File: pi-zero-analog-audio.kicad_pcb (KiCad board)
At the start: 2 copper layers, 65 x 30 mm, 40 parts, among them J1 GPIO, J2 Screw_Terminal_01x04, J3 Audio Jack, U1 MIC5365-3.3YD5, U2 MC74VHC1GT50, U3 MC74VHC1GT50, U4 PAM8403D

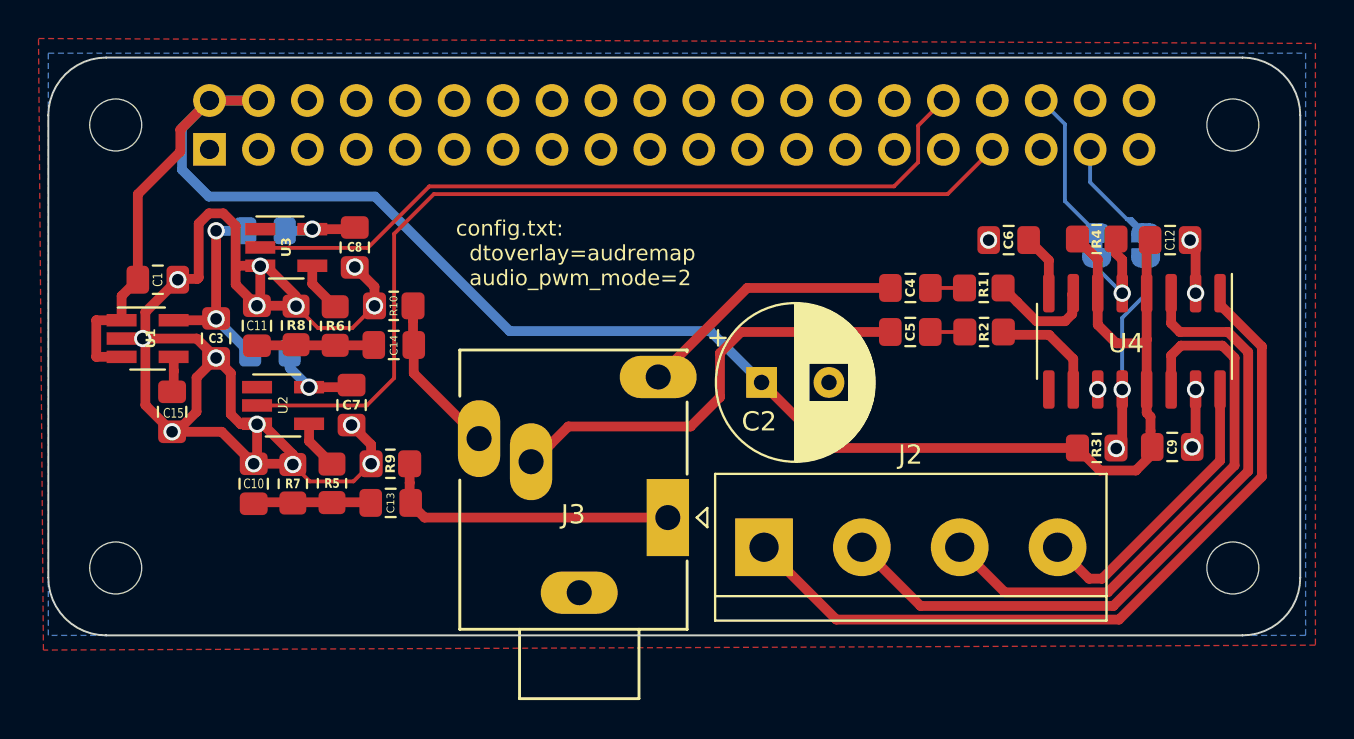
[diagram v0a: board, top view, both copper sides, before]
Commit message: Revert "Two GND zones"
This reverts commit edaad1ef0305b16592a24cacb57811a0cb0df8b8.
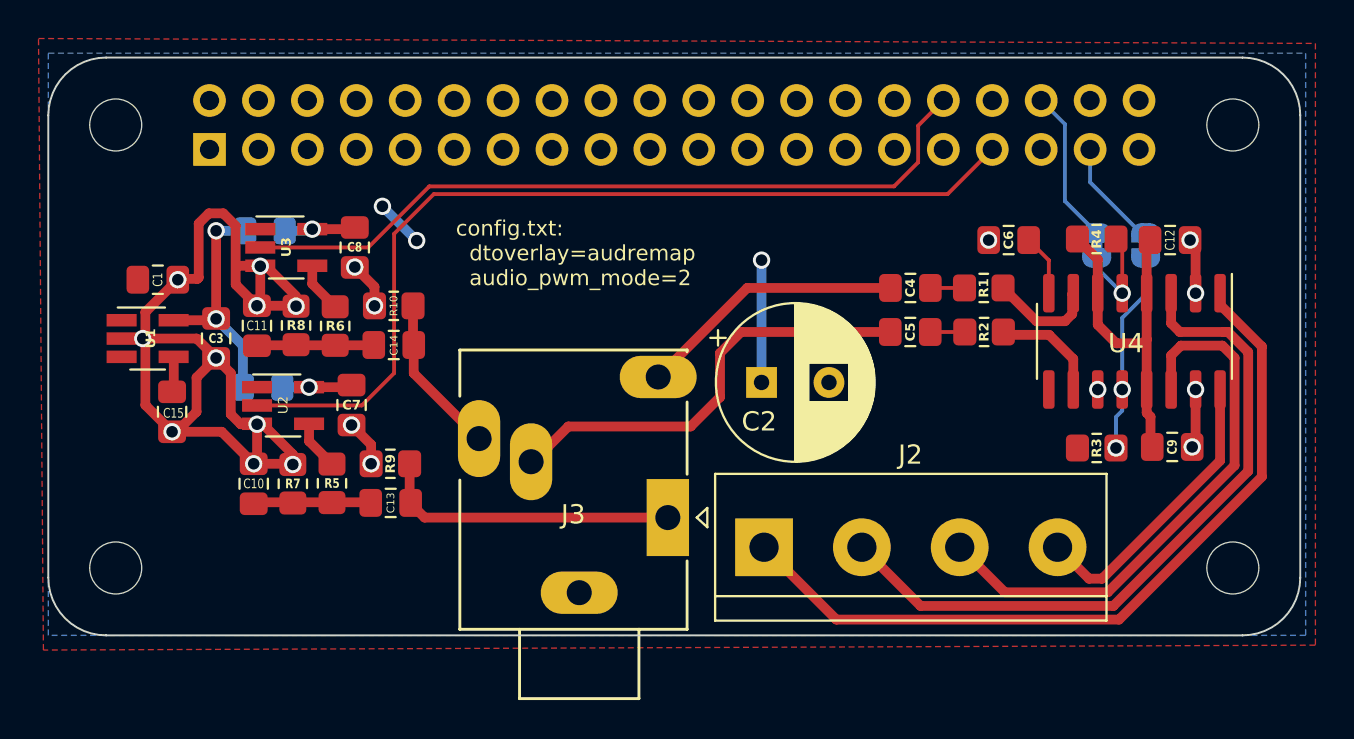
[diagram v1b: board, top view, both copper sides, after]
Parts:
- moved FB1 1.82 mm to (111.1, 87.1)
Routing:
- net +5V: track 103.7 -> 27.3 mm, vias 0 -> 3
- net GND: track 72.6 -> 63.0 mm
- net Net-(JP1-B): track 13.2 -> 10.5 mm
- net Net-(C10-Pad1): track 8.04 -> 6.04 mm
- net /AUD_3V3: track 10.7 -> 12.2 mm
- net /SHDN: track 6.69 -> 5.42 mm
- net Net-(U4-INL): track 6.63 -> 5.60 mm
- net Net-(U2-VCC): track 4.28 -> 3.26 mm
- net Net-(U1-NC): track 2.72 -> 1.99 mm
- net /AUDIO_L: track 16.2 -> 15.6 mm
- added copper zone on F.Cu, net +5V
